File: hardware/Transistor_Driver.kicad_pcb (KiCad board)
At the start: 2 copper layers, 35 x 45 mm, 11 parts, among them J1 Conn_GND, J2 Power_Output, J3 Conn_5V, K2 G5LE-1, Q2 BC547

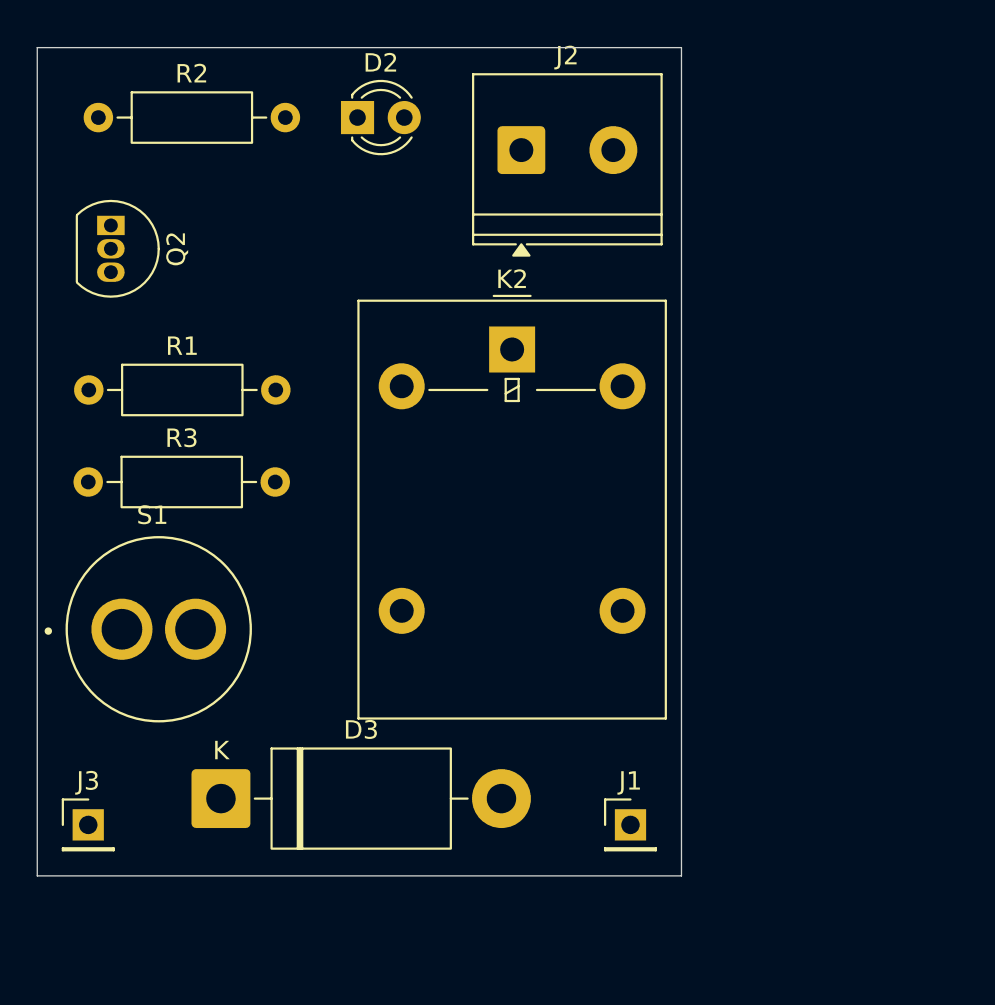
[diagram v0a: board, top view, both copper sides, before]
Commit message: feat(hardware): add PCB design
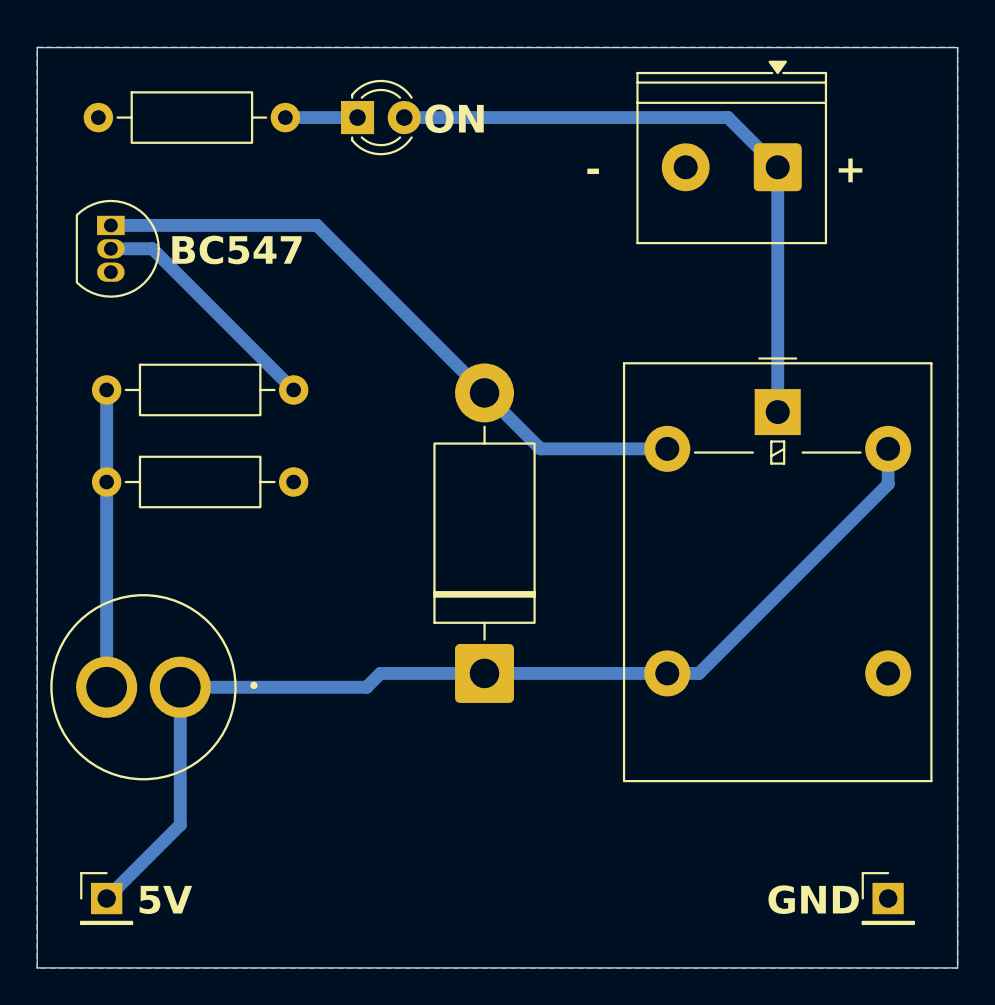
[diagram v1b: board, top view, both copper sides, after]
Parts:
- R3: renamed from R2; value 200 -> 220
- moved D1 15.9 mm to (199.5, 86.0), turned to 90 degrees
- moved K1 14.8 mm to (215.4, 71.8)
- moved J2 14.6 mm to (221.4, 98.2)
- moved J3 14.0 mm to (215.4, 58.5), turned to 180 degrees
- moved J1 4.12 mm to (179.0, 98.2)
- moved S1 3.26 mm to (181.0, 86.8), turned to 180 degrees
- moved R1 1.00 mm to (179.0, 75.6)
- moved R2 0.97 mm to (179.0, 70.6)
- renumbered D3 to D1, J3 to J1, J1 to J2, J2 to J3, K2 to K1, Q2 to Q1, R3 to R1, R1 to R2
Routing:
- net +5V: track 0.00 -> 58.1 mm
- net Net-(D1-A): track 0.00 -> 35.3 mm
- net Net-(D2-A): track 0.00 -> 34.7 mm
- net Net-(R1-Pad1): track 0.00 -> 16.2 mm
- net Net-(Q1-B): track 0.00 -> 13.1 mm
- net Net-(D2-K): track 0.00 -> 3.92 mm
- added copper zone on B.Cu, net GND
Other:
- board size 35 x 45 mm -> 50 x 50 mm
- board text added: "+"
- board text added: "-"
- board text added: "5V"
- board text added: "BC547"
- board text added: "GND"
- board text added: "ON"
